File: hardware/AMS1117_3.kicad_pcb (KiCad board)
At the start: 2 copper layers, 9 parts, among them J14 Va_header, U6 AMS1117-3.3

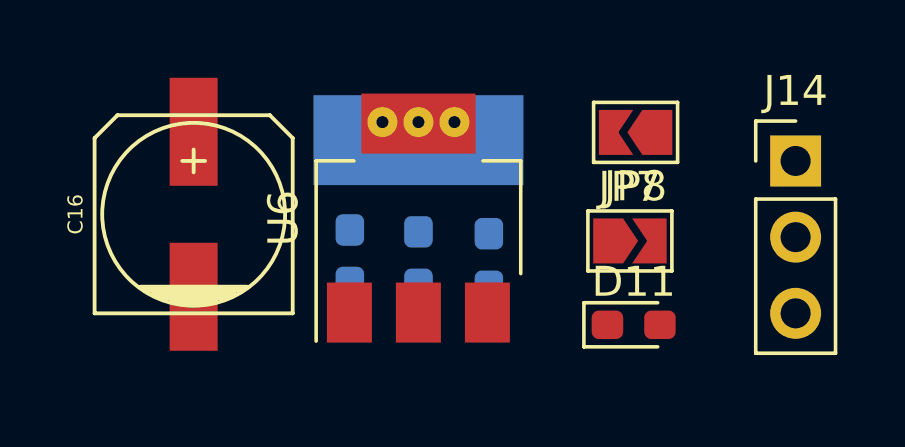
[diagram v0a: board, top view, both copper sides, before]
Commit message: update,
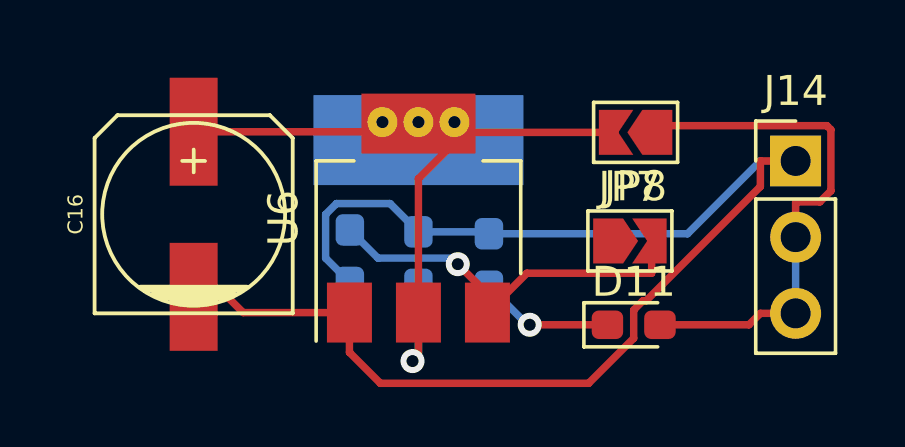
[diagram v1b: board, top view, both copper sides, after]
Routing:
- net GND: track 0.00 -> 46.0 mm
- net Net-(C15-Pad1): track 0.00 -> 25.3 mm, vias 0 -> 1
- net Vc: track 0.00 -> 17.7 mm
- net Net-(C14-Pad1): track 0.00 -> 13.0 mm, vias 0 -> 1
- net Net-(D11-Pad1): track 0.00 -> 4.48 mm, vias 0 -> 1
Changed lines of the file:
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@@
     (thickness 1.6)
     (drawings 0)
-    (tracks 0)
+    (tracks 62)
     (zones 0)
     (modules 9)
@@
     (uvia_dia 0.3)
     (uvia_drill 0.1)
-    (add_net +5V)
     (add_net GND)
     (add_net "Net-(C14-Pad1)")
@@
     )
   )
+  (segment (start 22.6695 19.8895) (end 24.9555 19.8895) (width 0.25) (layer B.Cu) (net 1))
+  (segment (start 24.9555 19.8895) (end 25.019 19.953) (width 0.25) (layer B.Cu) (net 1))
+  (segment (start 20.3835 21.576) (end 19.576 20.7685) (width 0.25) (layer B.Cu) (net 1))
+  (segment (start 19.576 20.7685) (end 19.576 19.3076) (width 0.25) (layer B.Cu) (net 1))
+  (segment (start 19.576 19.3076) (end 19.9367 18.9469) (width 0.25) (layer B.Cu) (net 1))
+  (segment (start 19.9367 18.9469) (end 21.7269 18.9469) (width 0.25) (layer B.Cu) (net 1))
+  (segment (start 21.7269 18.9469) (end 22.6695 19.8895) (width 0.25) (layer B.Cu) (net 1))
+  (segment (start 35.2425 17.526) (end 34.0672 17.526) (width 0.25) (layer B.Cu) (net 1))
+  (segment (start 34.0672 17.526) (end 31.6402 19.953) (width 0.25) (layer B.Cu) (net 1))
+  (segment (start 31.6402 19.953) (end 25.019 19.953) (width 0.25) (layer B.Cu) (net 1))
+  (segment (start 15.1765 22.0548) (end 16.3019 22.0548) (width 0.25) (layer F.Cu) (net 1))
+  (segment (start 16.3019 22.0548) (end 16.8281 22.581) (width 0.25) (layer F.Cu) (net 1))
+  (segment (start 16.8281 22.581) (end 20.3695 22.581) (width 0.25) (layer F.Cu) (net 1))
+  (segment (start 20.3695 22.581) (end 20.3695 23.9063) (width 0.25) (layer F.Cu) (net 1))
+  (segment (start 20.3695 23.9063) (end 21.4006 24.9374) (width 0.25) (layer F.Cu) (net 1))
+  (segment (start 21.4006 24.9374) (end 28.3433 24.9374) (width 0.25) (layer F.Cu) (net 1))
+  (segment (start 28.3433 24.9374) (end 29.845 23.4357) (width 0.25) (layer F.Cu) (net 1))
+  (segment (start 29.845 23.4357) (end 29.845 22.4943) (width 0.25) (layer F.Cu) (net 1))
+  (segment (start 29.845 22.4943) (end 30.1536 22.1857) (width 0.25) (layer F.Cu) (net 1))
+  (segment (start 30.1536 22.1857) (end 30.2609 22.1857) (width 0.25) (layer F.Cu) (net 1))
+  (segment (start 30.2609 22.1857) (end 34.0672 18.3794) (width 0.25) (layer F.Cu) (net 1))
+  (segment (start 34.0672 18.3794) (end 34.0672 17.526) (width 0.25) (layer F.Cu) (net 1))
+  (segment (start 35.2425 17.526) (end 34.0672 17.526) (width 0.25) (layer F.Cu) (net 1))
+  (segment (start 25.2827 22.2678) (end 23.9807 20.9659) (width 0.25) (layer F.Cu) (net 2))
+  (segment (start 20.3835 19.826) (end 21.322 20.7645) (width 0.25) (layer B.Cu) (net 2))
+  (segment (start 21.322 20.7645) (end 23.7793 20.7645) (width 0.25) (layer B.Cu) (net 2))
+  (segment (start 23.7793 20.7645) (end 23.9807 20.9659) (width 0.25) (layer B.Cu) (net 2))
+  (segment (start 25.2827 22.2678) (end 24.9695 22.581) (width 0.25) (layer F.Cu) (net 2))
+  (segment (start 30.443 21.2683) (end 26.2822 21.2683) (width 0.25) (layer F.Cu) (net 2))
+  (segment (start 26.2822 21.2683) (end 25.2827 22.2678) (width 0.25) (layer F.Cu) (net 2))
+  (segment (start 30.443 20.193) (end 30.443 21.2683) (width 0.25) (layer F.Cu) (net 2))
+  (via (at 23.9807 20.9659) (size 0.8) (layers F.Cu B.Cu) (net 2))
+  (segment (start 22.6695 22.581) (end 22.6695 23.9063) (width 0.25) (layer F.Cu) (net 3))
+  (segment (start 22.6695 23.9063) (end 22.4726 24.1032) (width 0.25) (layer F.Cu) (net 3))
+  (segment (start 22.4726 24.1032) (end 22.4726 24.1967) (width 0.25) (layer F.Cu) (net 3))
+  (segment (start 24.212 16.5735) (end 22.6695 18.116) (width 0.25) (layer F.Cu) (net 3))
+  (segment (start 22.6695 18.116) (end 22.6695 22.581) (width 0.25) (layer F.Cu) (net 3))
+  (segment (start 22.4726 24.1967) (end 22.6695 23.9998) (width 0.25) (layer B.Cu) (net 3))
+  (segment (start 22.6695 23.9998) (end 22.6695 21.6395) (width 0.25) (layer B.Cu) (net 3))
+  (segment (start 24.212 16.5735) (end 23.8695 16.231) (width 0.25) (layer F.Cu) (net 3))
+  (segment (start 29.1835 16.5735) (end 24.212 16.5735) (width 0.25) (layer F.Cu) (net 3))
+  (segment (start 22.6695 16.231) (end 23.8695 16.231) (width 0.25) (layer F.Cu) (net 3))
+  (segment (start 21.4695 16.231) (end 22.6695 16.231) (width 0.25) (layer F.Cu) (net 3))
+  (segment (start 22.6695 16.281) (end 22.6695 16.231) (width 0.25) (layer F.Cu) (net 3))
+  (segment (start 15.1765 16.5532) (end 21.1473 16.5532) (width 0.25) (layer F.Cu) (net 3))
+  (segment (start 21.1473 16.5532) (end 21.4695 16.231) (width 0.25) (layer F.Cu) (net 3))
+  (via (at 22.4726 24.1967) (size 0.8) (layers F.Cu B.Cu) (net 3))
+  (segment (start 35.2425 20.066) (end 35.2425 18.8907) (width 0.25) (layer F.Cu) (net 4))
+  (segment (start 35.2425 18.8907) (end 36.0505 18.8907) (width 0.25) (layer F.Cu) (net 4))
+  (segment (start 36.0505 18.8907) (end 36.4179 18.5233) (width 0.25) (layer F.Cu) (net 4))
+  (segment (start 36.4179 18.5233) (end 36.4179 16.4834) (width 0.25) (layer F.Cu) (net 4))
+  (segment (start 36.4179 16.4834) (end 36.2851 16.3506) (width 0.25) (layer F.Cu) (net 4))
+  (segment (start 36.2851 16.3506) (end 30.8564 16.3506) (width 0.25) (layer F.Cu) (net 4))
+  (segment (start 30.8564 16.3506) (end 30.6335 16.5735) (width 0.25) (layer F.Cu) (net 4))
+  (segment (start 35.2425 20.066) (end 35.2425 22.606) (width 0.25) (layer B.Cu) (net 4))
+  (segment (start 35.2425 22.606) (end 34.0672 22.606) (width 0.25) (layer F.Cu) (net 4))
+  (segment (start 30.72 22.987) (end 33.6862 22.987) (width 0.25) (layer F.Cu) (net 4))
+  (segment (start 33.6862 22.987) (end 34.0672 22.606) (width 0.25) (layer F.Cu) (net 4))
+  (segment (start 28.97 22.987) (end 26.3781 22.987) (width 0.25) (layer F.Cu) (net 5))
+  (segment (start 25.019 21.703) (end 26.303 22.987) (width 0.25) (layer B.Cu) (net 5))
+  (segment (start 26.303 22.987) (end 26.3781 22.987) (width 0.25) (layer B.Cu) (net 5))
+  (via (at 26.3781 22.987) (size 0.8) (layers F.Cu B.Cu) (net 5))
 )
